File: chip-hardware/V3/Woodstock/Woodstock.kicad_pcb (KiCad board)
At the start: 2 copper layers, 16.5 x 19.1 mm, 11 parts, among them J1 501461-0491, U1 MCP9808_MSOP, U2 LIS3DH

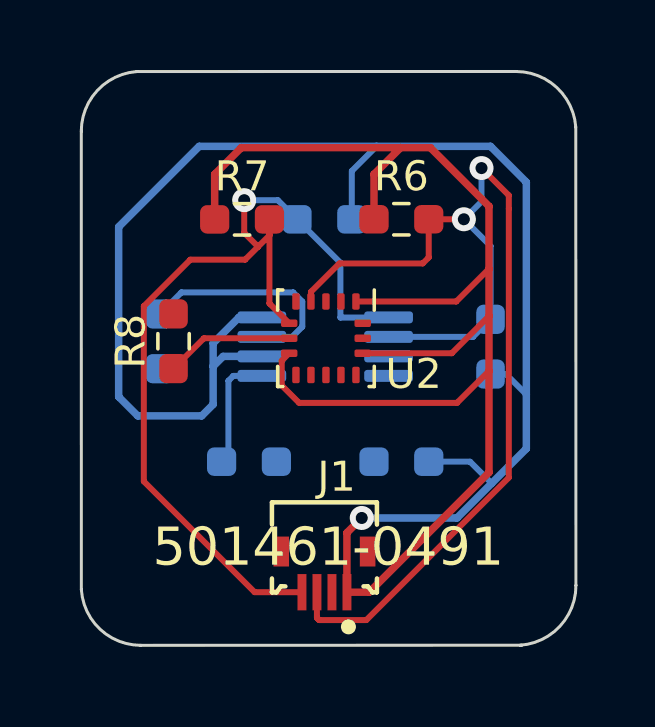
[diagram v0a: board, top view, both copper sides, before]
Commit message: Connceted everything that needs to be connected. Looks good
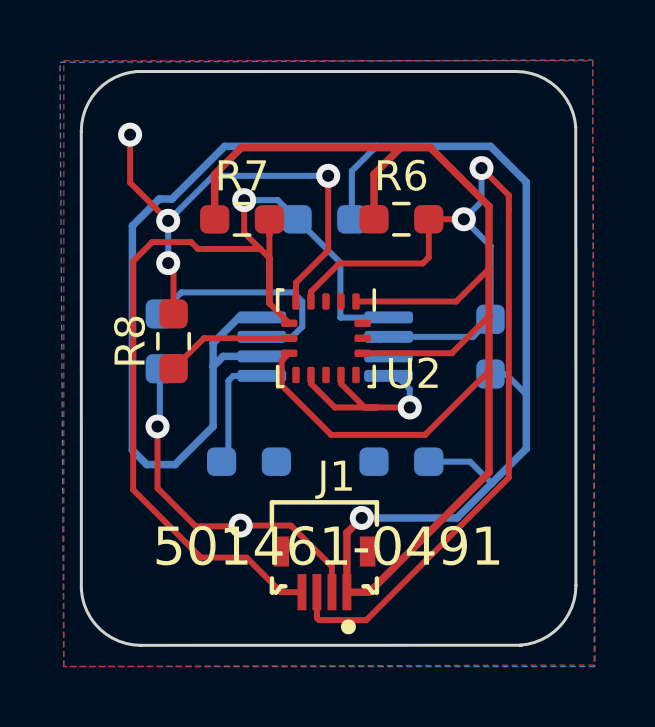
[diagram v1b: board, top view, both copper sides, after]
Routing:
- net GND: track 0.00 -> 36.1 mm, vias 0 -> 7
- net /SDA: track 31.3 -> 34.8 mm
- net +3V3: track 103.1 -> 105.9 mm
- added copper zone on B.Cu, net GND
- added copper zone on F.Cu, net GND
